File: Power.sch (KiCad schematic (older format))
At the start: 31 parts, among them J2 FAN, J3 PWR, Q1 IRFML8244, Q2 AOD4189, Q3 AOD4189, Q4 MMBT3906, Q5 MMBT3904, Q6 MMBT3904

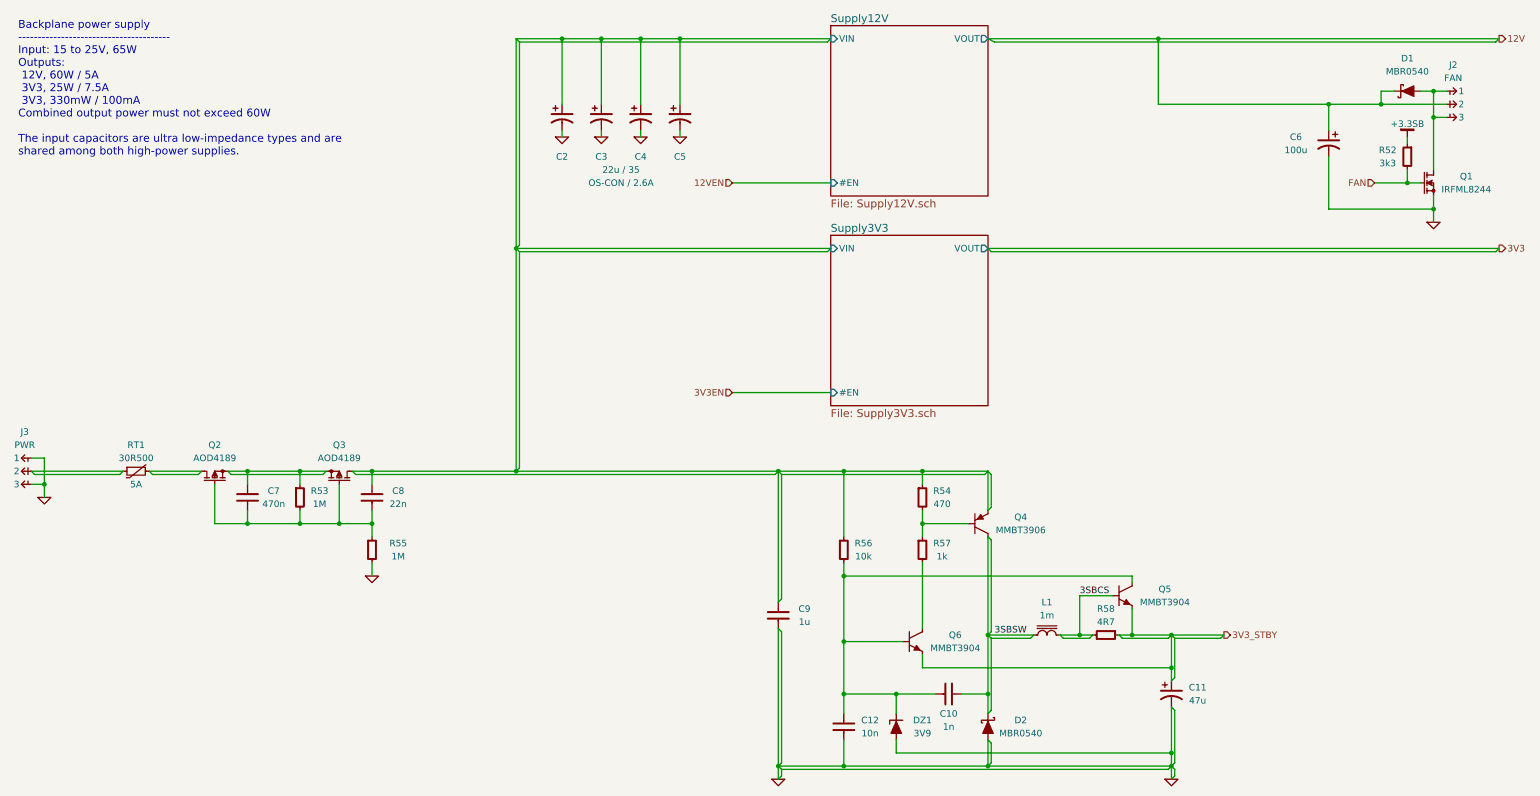
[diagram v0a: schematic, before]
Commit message: Silkscreen and 3D touchups
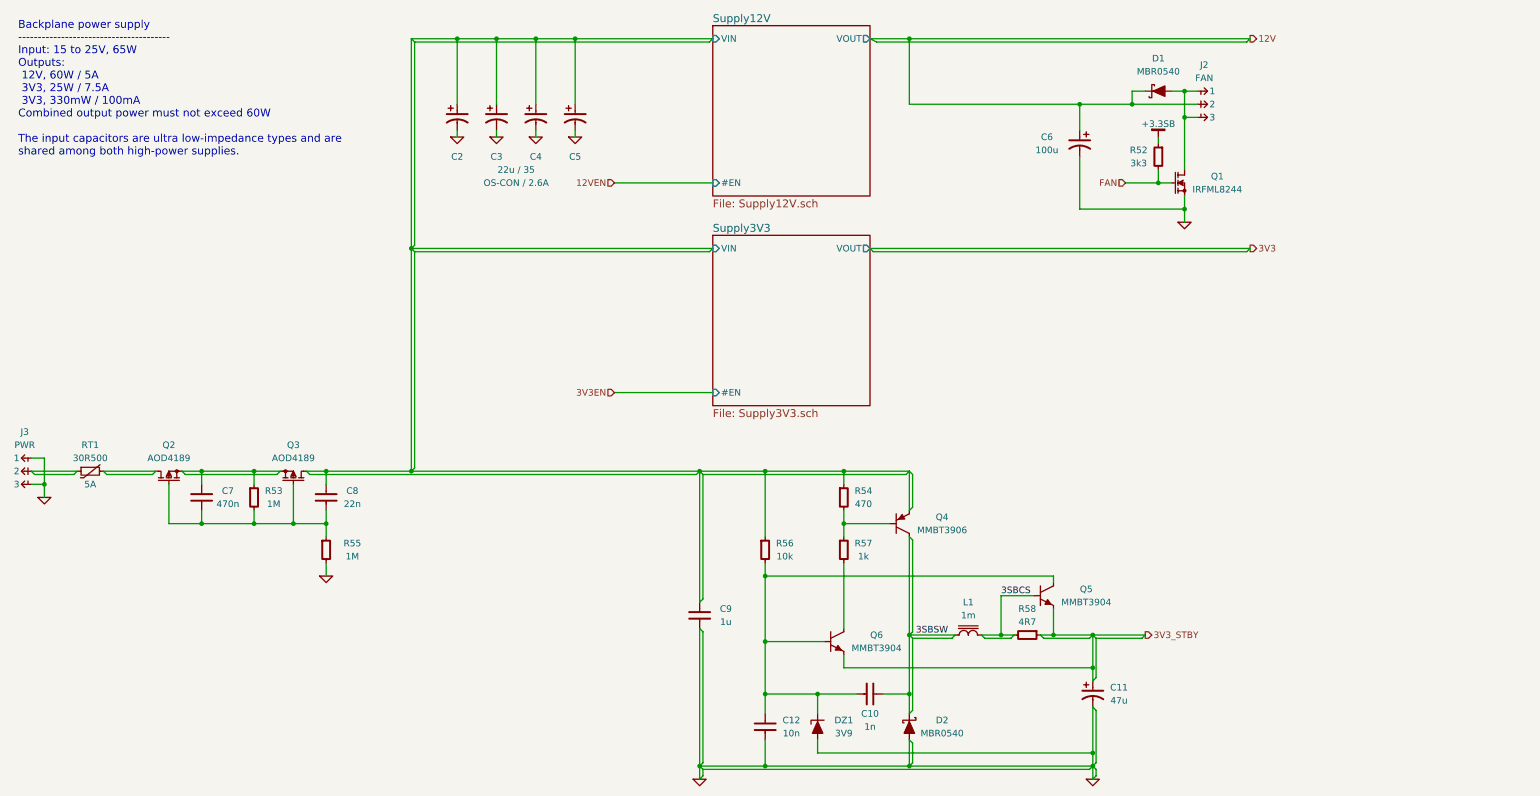
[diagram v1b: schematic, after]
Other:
- moved on the sheet: C10, C11, C12, C2, C3, C4, C5, C6, C7, C8, C9, D1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
